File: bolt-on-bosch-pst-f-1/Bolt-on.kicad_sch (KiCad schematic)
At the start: 10 parts

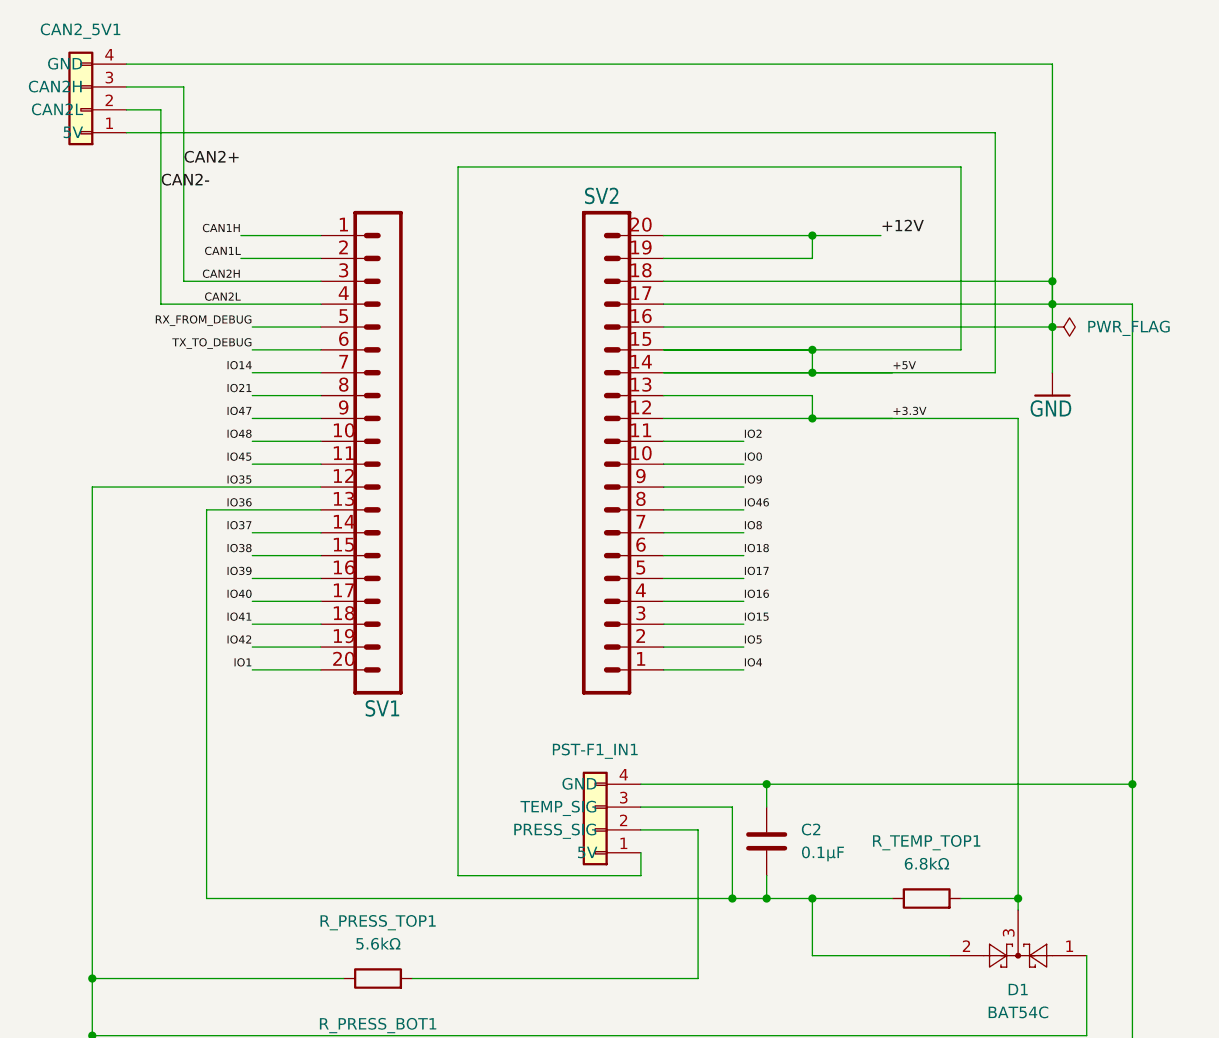
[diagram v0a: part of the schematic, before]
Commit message: swaped jst positions
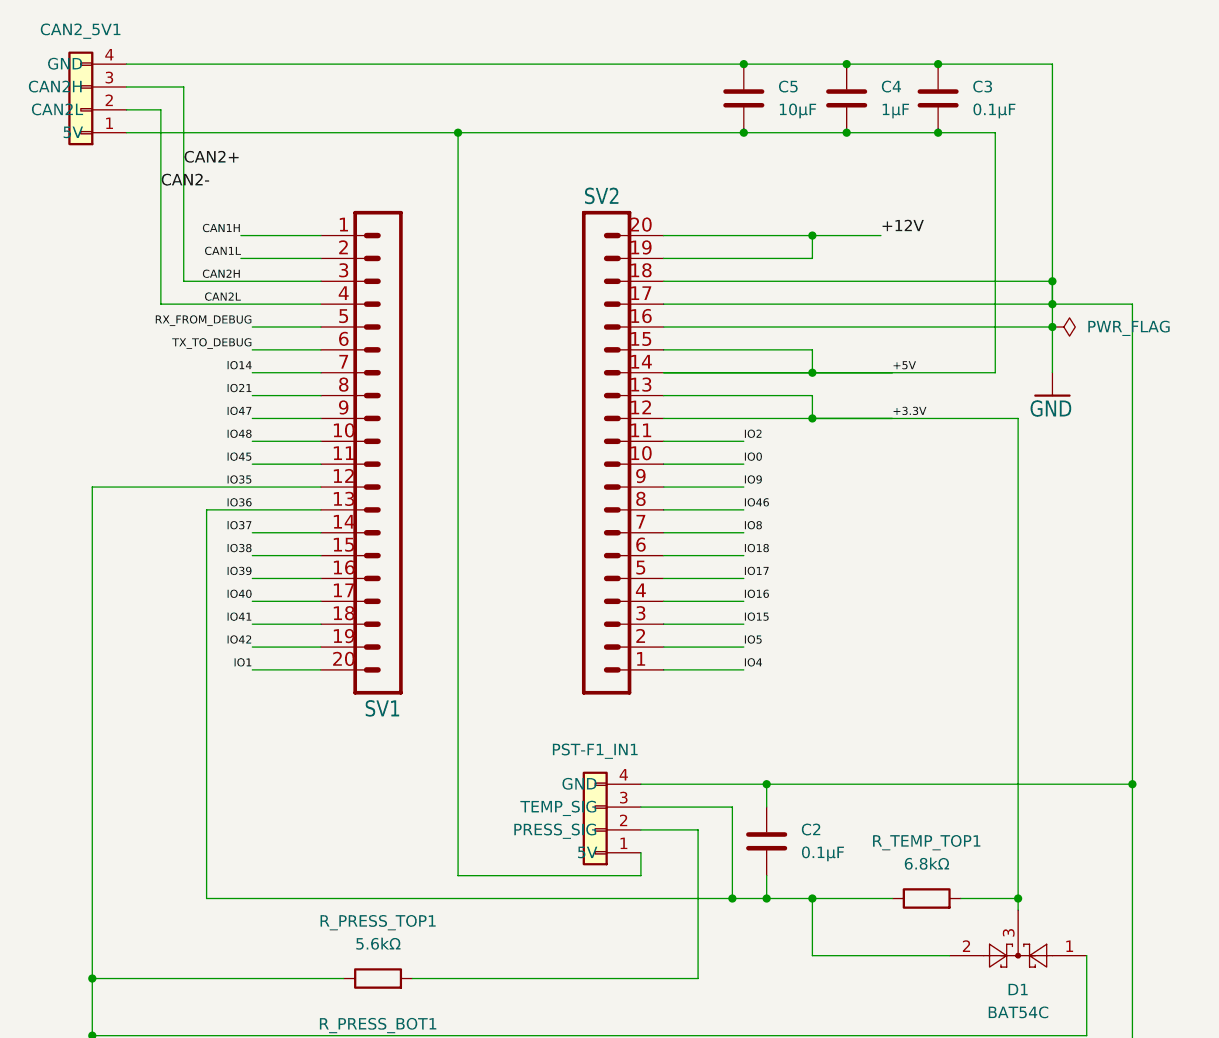
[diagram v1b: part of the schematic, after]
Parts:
- added C3: ﻿0.1µF, Capacitor_SMD:C_0805_2012Metric_Pad1.18x1.45mm_HandSolder, symbol Device:C
- added C4: 1µF, Capacitor_SMD:C_0805_2012Metric_Pad1.18x1.45mm_HandSolder, symbol Device:C
- added C5: 10µF, Capacitor_SMD:C_1206_3216Metric_Pad1.33x1.80mm_HandSolder, symbol Device:C
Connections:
- net +5V: now also C3.2, C4.2, C5.2
- net GND: now also C3.1, C4.1, C5.1
